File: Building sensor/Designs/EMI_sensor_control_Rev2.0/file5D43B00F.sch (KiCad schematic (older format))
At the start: 12 parts, among them U14 AD8021ARZ

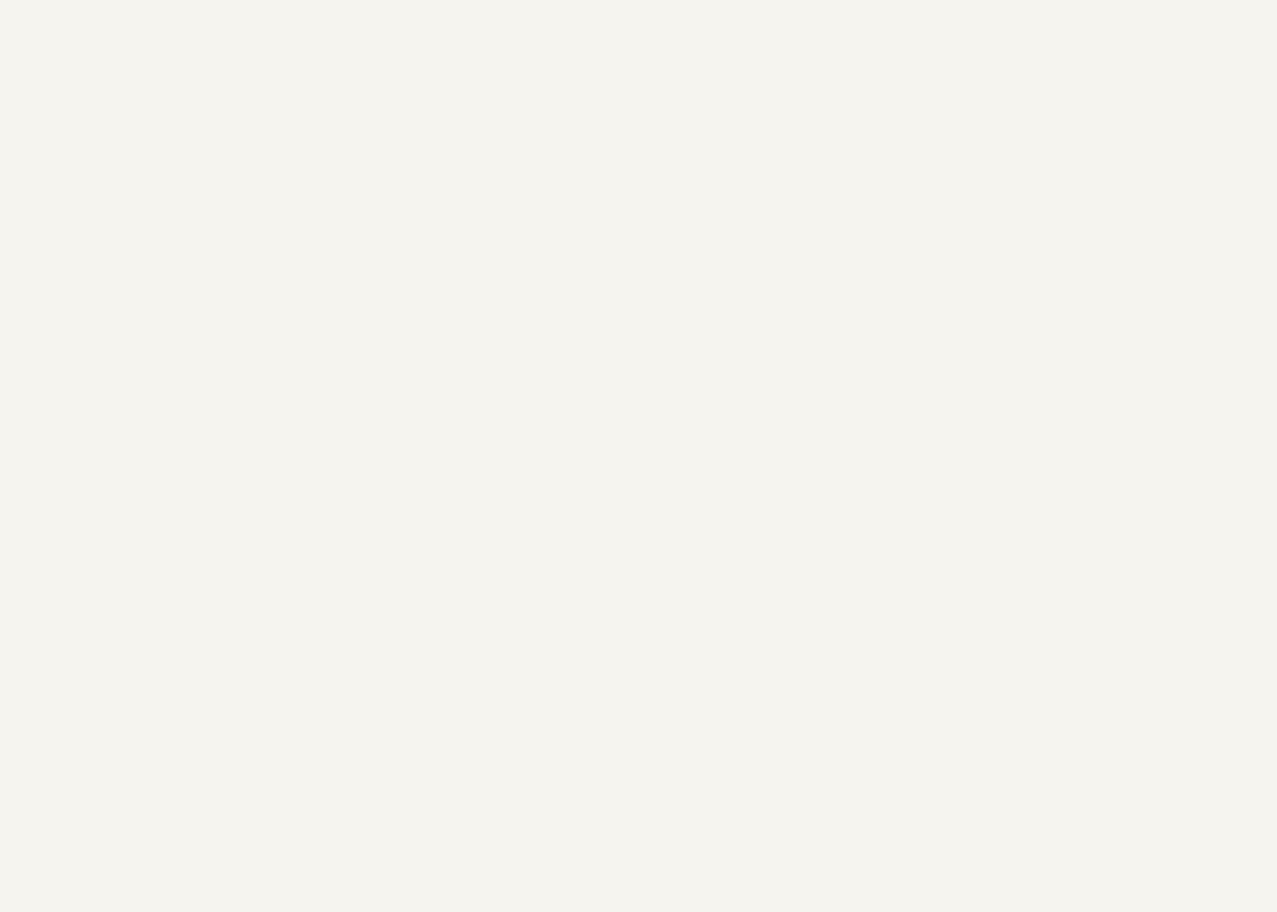
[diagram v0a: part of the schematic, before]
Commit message: backup
2/04/2020
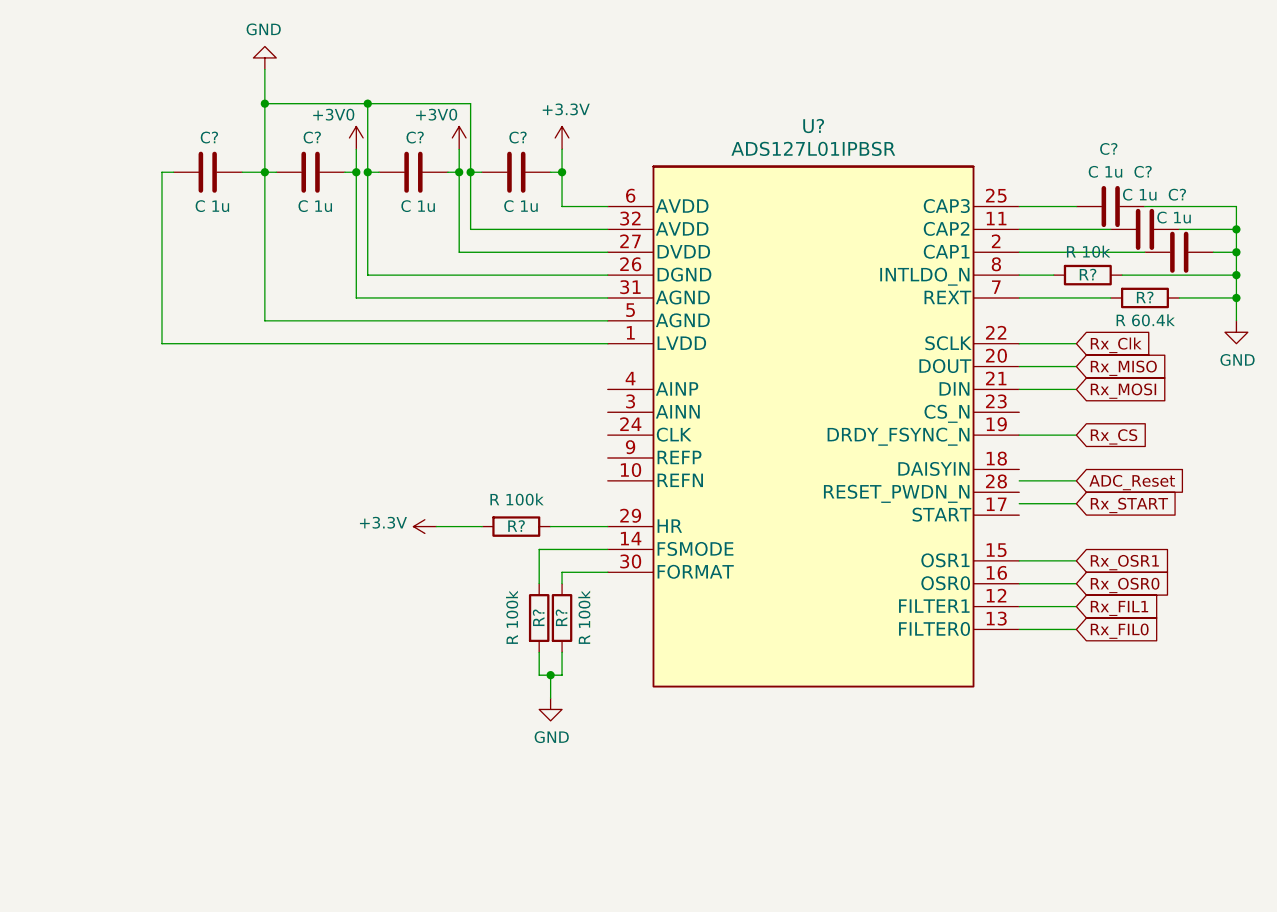
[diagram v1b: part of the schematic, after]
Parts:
- added C? (x7): C 1u, Capacitor_SMD:C_0402_1005Metric, symbol Device:C
- added R? (x3): R 100k, Resistor_SMD:R_0805_2012Metric_Pad1.15x1.40mm_HandSolder, symbol Device:R
- added R?: R 10k, Resistor_SMD:R_0805_2012Metric_Pad1.15x1.40mm_HandSolder, symbol Device:R
- added R?: R 60.4k, Resistor_SMD:R_0805_2012Metric_Pad1.15x1.40mm_HandSolder, symbol Device:R
- added U?: ADS127L01IPBSR, PBS0032A_N, symbol 2019-12-03_16-41-56:ADS127L01IPBSR
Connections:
- net GND: now also C?.1, C?.1, C?.1, C?.1, C?.1, C?.1, C?.2, R?.1, R?.1, R?.2, R?.2, U?.26 (DGND), U?.32 (AVDD), U?.5 (AGND)
- new net: C?.1, U?.1 (LVDD)
- new net: C?.2, U?.11 (CAP2)
- new net: R?.1, U?.14 (FSMODE)
- new net: C?.2, U?.2 (CAP1)
- new net: C?.2, U?.25 (CAP3)
- new net: R?.1, U?.29 (HR)
- new net: R?.1, U?.30 (FORMAT)
- new net: R?.2, U?.7 (REXT)
- new net: R?.2, U?.8 (INTLDO_N)
- new net +3V0: C?.2, C?.2, U?.27 (DVDD), U?.31 (AGND)
- new net +3V3: C?.2, R?.2, U?.6 (AVDD)
- new net Rx_CS: U?.19 (DRDY_FSYNC_N)
- new net Rx_Clk: U?.22 (SCLK)
- new net Rx_FIL0: U?.13 (FILTER0)
- new net Rx_FIL1: U?.12 (FILTER1)
- new net Rx_MISO: U?.20 (DOUT)
- new net Rx_MOSI: U?.21 (DIN)
- new net Rx_OSR0: U?.16 (OSR0)
- new net Rx_OSR1: U?.15 (OSR1)
